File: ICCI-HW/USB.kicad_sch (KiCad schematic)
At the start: 25 parts, among them J201 USB_C_Receptacle_USB2.0, Q201 PDTC114Y, Q202 PDTC114Y, U201 CP2102N-Axx-xQFN28

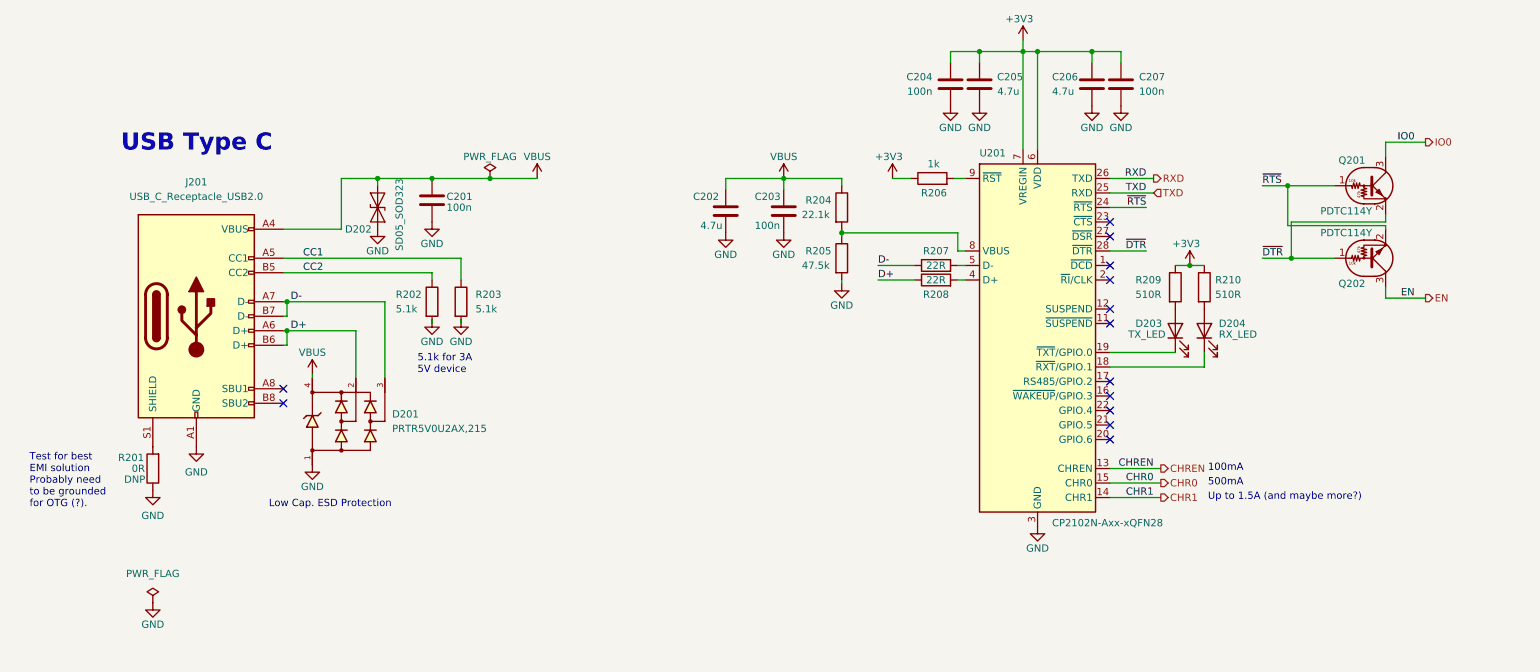
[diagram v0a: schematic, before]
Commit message: hw: updates
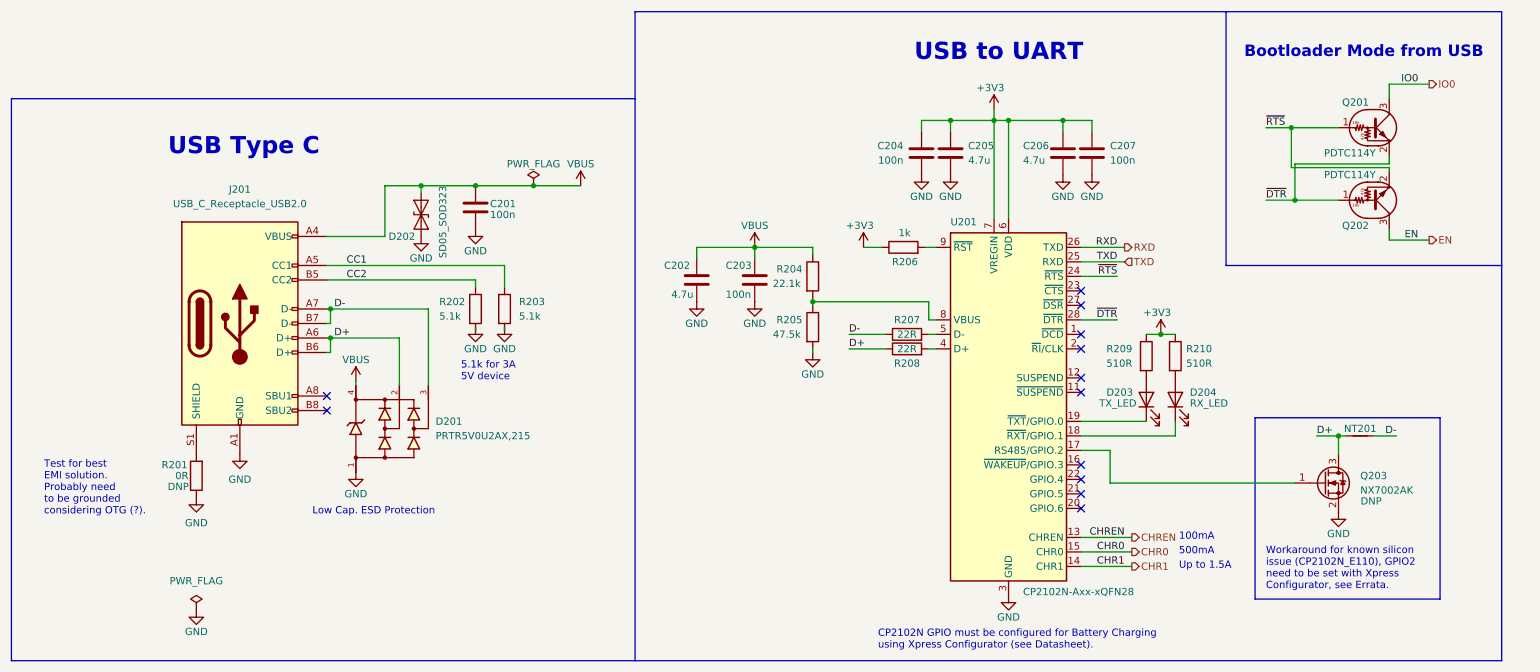
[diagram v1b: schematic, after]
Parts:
- added NT201: NetTie_2, NetTie:NetTie-2_SMD_Pad0.5mm, symbol Device:NetTie_2
- added Q203: NX7002AK, Package_TO_SOT_SMD:SOT-23, symbol Device:Q_NMOS_GSD
- R201: now in the parts list
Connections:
- net D+: now also NT201.1, Q203.3 (D)
- net D-: now also NT201.2
- net GND: now also Q203.2 (S)
- net at U201.17 (RS485/GPIO.2): now also Q203.1 (G)
- no-connect marks 13 -> 12
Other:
- note added: "Bootloader Mode from USB"
- note added: "CP2102N GPIO must be configured for Battery Charging using Xpress Configurator (see Datasheet)."
- note added: "Test for best EMI solution. Probably need to be grounded considering OTG (?)."
- note added: "USB to UART"
- note added: "Up to 1.5A"
- note added: "Workaround for known silicon issue (CP2102N_E110), GPIO2 need to be set with Xpress Configurator, see Errata."
- note removed: "Test for best EMI solution Probably need to be grounded for OTG (?)."
- note removed: "Up to 1.5A (and maybe more?)"
- company: tollsimy -> Simone Tollardo
- moved on the sheet: C201, C202, C203, C204, C205, C206, C207, D201, D202, D203, D204, J201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
